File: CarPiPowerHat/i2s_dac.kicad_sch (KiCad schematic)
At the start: 23 parts, among them J4 AudioJack2_Ground, Q3 DMG2305, U5 AP2112-3.3K, U6 UDA1334ATS

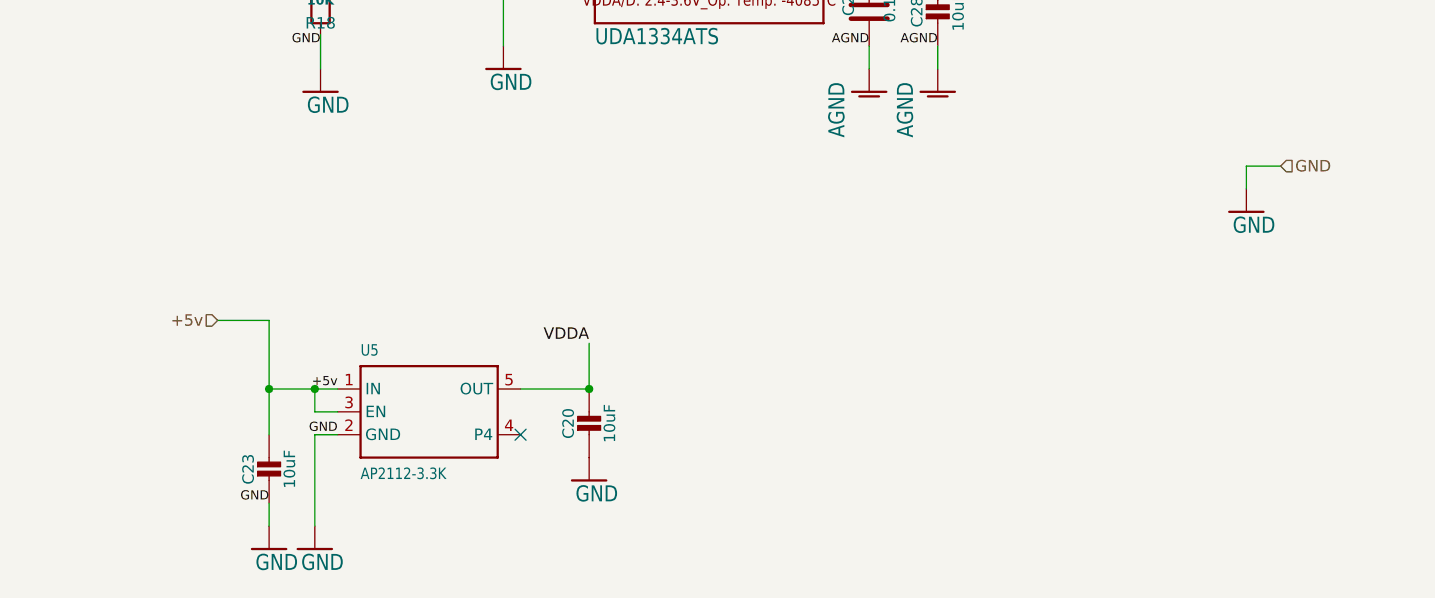
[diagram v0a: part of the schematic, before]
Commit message: Finalized 2.2
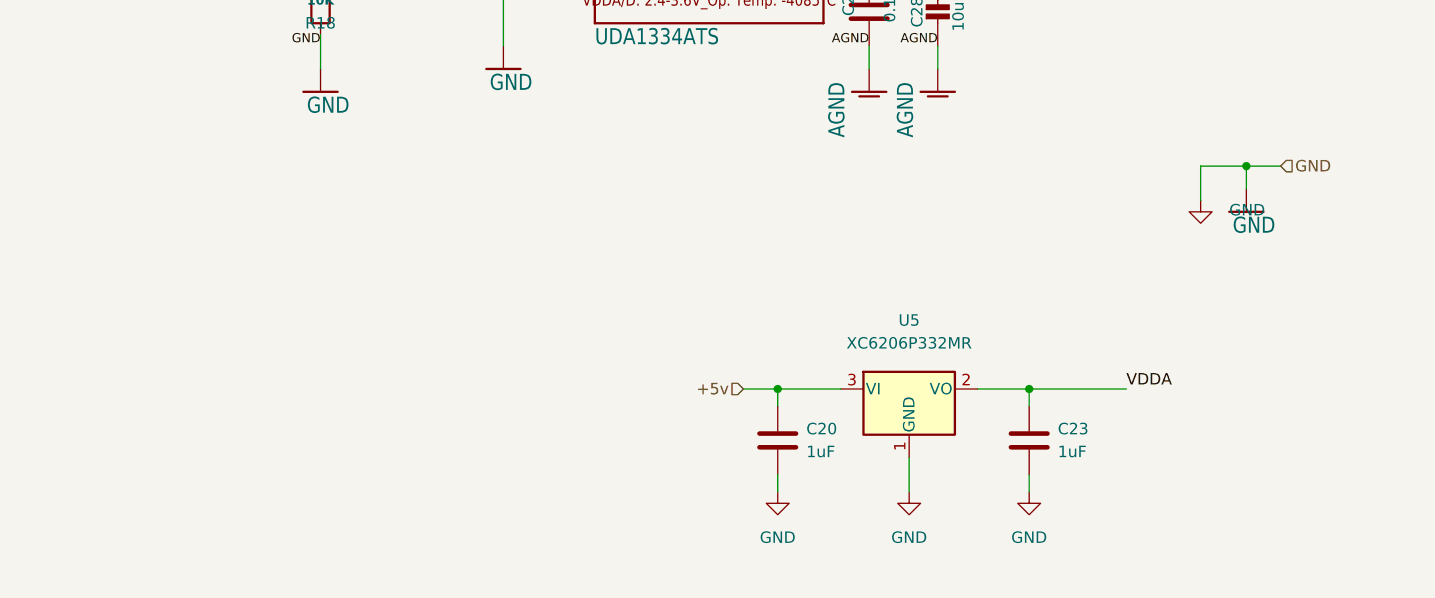
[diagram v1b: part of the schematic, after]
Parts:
- removed C20, C23: 10uF, Capacitor_SMD:C_0805_2012Metric, symbol Adafruit I2S Audio UDA1334 Bonnet-eagle-import:CAP_CERAMIC0805-NOOUTLINE
- removed U5: AP2112-3.3K, Package_TO_SOT_SMD:SOT-23-5_HandSoldering, symbol Adafruit I2S Audio UDA1334 Bonnet-eagle-import:VREG_SOT23-5
- added C20, C23: 1uF, Capacitor_SMD:C_0805_2012Metric_Pad1.18x1.45mm_HandSolder, symbol Device:C
- added U5: XC6206P332MR, Package_TO_SOT_SMD:SOT-23, symbol Regulator_Linear:XC6206PxxxMR
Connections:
- net +5v: now also C20.1, U5.3 (VI)
- net GND: now also C20.2, C23.2, U5.1 (GND)
- net VDDA: now also C23.1, U5.2 (VO)
- no-connect marks 1 -> 0
